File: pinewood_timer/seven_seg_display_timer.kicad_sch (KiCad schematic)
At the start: 56 parts, among them M1 N-MOSFET, M10 N-MOSFET, M11 N-MOSFET, M12 N-MOSFET, M13 N-MOSFET, M14 N-MOSFET, M15 N-MOSFET, M16 N-MOSFET, M2 N-MOSFET, M3 N-MOSFET, M4 N-MOSFET, M5 N-MOSFET, M6 N-MOSFET, M7 N-MOSFET, M8 N-MOSFET, M9 N-MOSFET, U2 TDCR1050M, U3 TDCR1050M, U4 TDCR1050M, U5 TDCR1050M, U6 74HC138, U7 74HC138, U8 TLC59210IN, U9 TLC59210IN

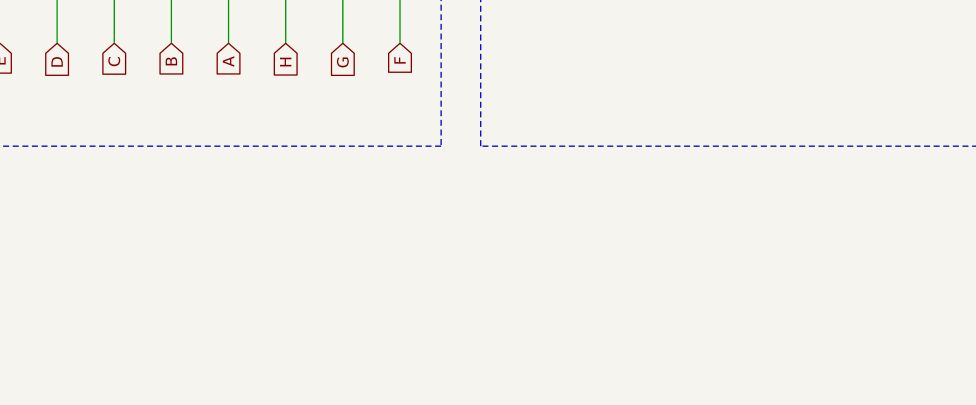
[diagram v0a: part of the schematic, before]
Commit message: added pins
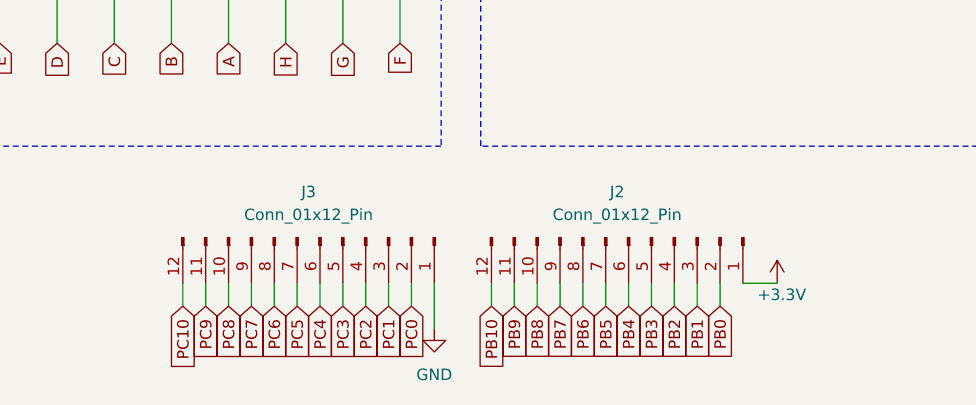
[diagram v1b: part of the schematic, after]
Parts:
- added J2, J3: Conn_01x12_Pin, symbol Connector:Conn_01x12_Pin
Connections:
- net +3.3V: now also J2.1 (Pin_1)
- net GND: now also J3.1 (Pin_1)
- net PB0: now also J2.2 (Pin_2)
- net PB1: now also J2.3 (Pin_3)
- net PB10: now also J2.12 (Pin_12)
- net PB2: now also J2.4 (Pin_4)
- net PB3: now also J2.5 (Pin_5)
- net PB4: now also J2.6 (Pin_6)
- net PB5: now also J2.7 (Pin_7)
- net PB6: now also J2.8 (Pin_8)
- net PB7: now also J2.9 (Pin_9)
- net PB8: now also J2.10 (Pin_10)
- net PB9: now also J2.11 (Pin_11)
- net PC0: now also J3.2 (Pin_2)
- net PC1: now also J3.3 (Pin_3)
- net PC10: now also J3.12 (Pin_12)
- net PC2: now also J3.4 (Pin_4)
- net PC3: now also J3.5 (Pin_5)
- net PC4: now also J3.6 (Pin_6)
- net PC5: now also J3.7 (Pin_7)
- net PC6: now also J3.8 (Pin_8)
- net PC7: now also J3.9 (Pin_9)
- net PC8: now also J3.10 (Pin_10)
- net PC9: now also J3.11 (Pin_11)
